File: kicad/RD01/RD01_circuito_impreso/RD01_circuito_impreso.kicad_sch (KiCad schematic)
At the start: 13 parts, among them P1 esp 35, P2 +Bat, P3 esp 26, P4 +Vcc, P5 bot encend, P6 GND, Q1 AO3401, Q2 AO3400

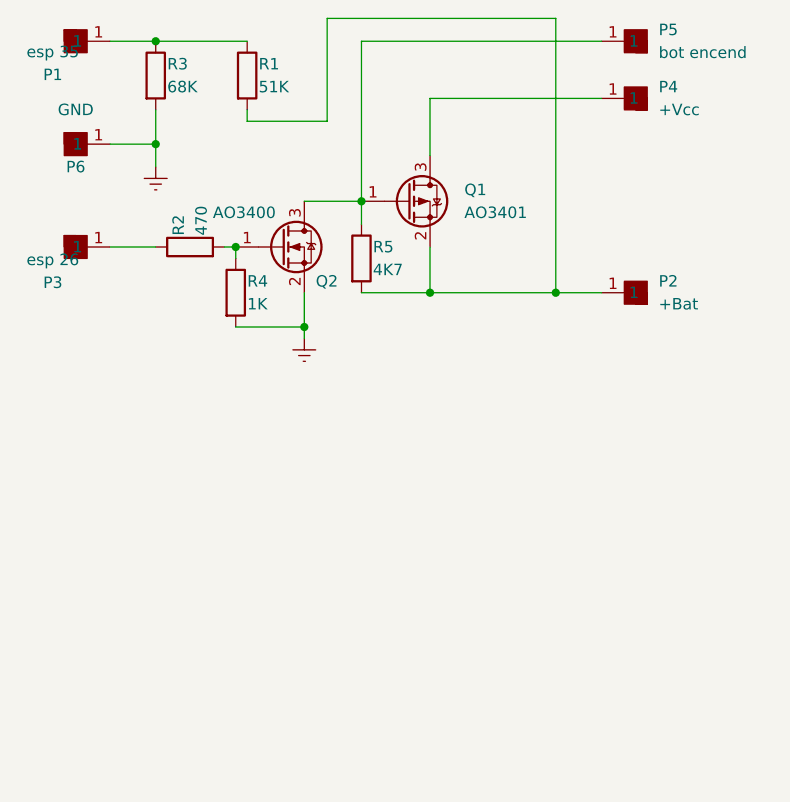
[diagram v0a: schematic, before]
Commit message: 9
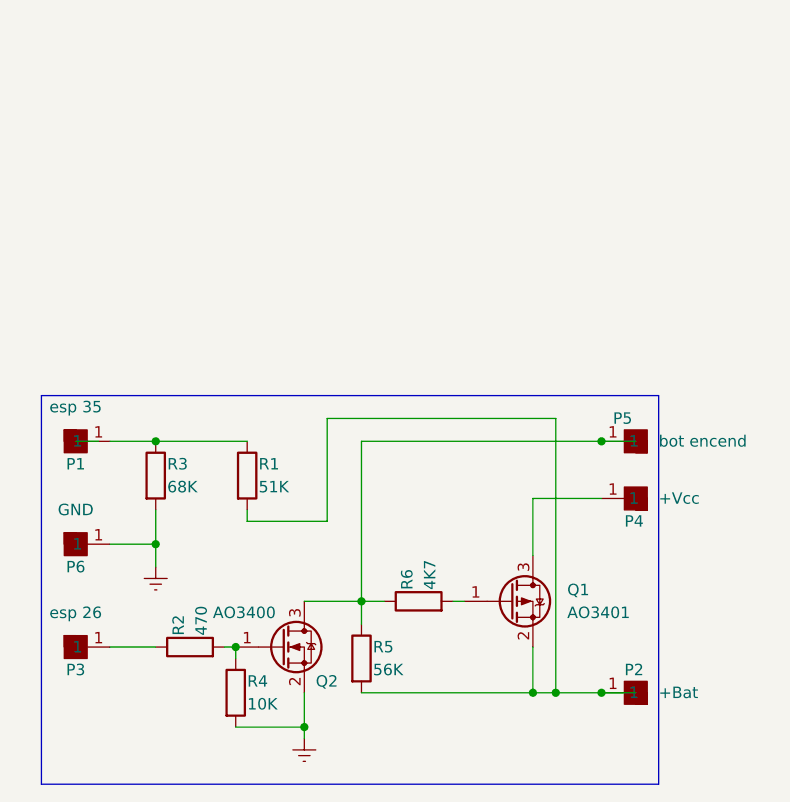
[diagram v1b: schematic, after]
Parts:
- added R6: 4K7, Resistor_THT:R_Axial_DIN0207_L6.3mm_D2.5mm_P10.16mm_Horizontal, symbol Device:R
- R4: value 1K -> 10K
- R5: value 4K7 -> 56K
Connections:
- net at P5.1, Q2.3 (D), R5.1: now also R6.1; no longer Q1.1 (G)
- new net: Q1.1 (G), R6.2
